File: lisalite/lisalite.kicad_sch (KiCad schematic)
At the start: 16 parts, among them J1 LisaLite FDD Connector, J2 LisaLite Twiggy Port Connector, U1 5MHz XTAL, U2 74LS74, U3 74LS393, U4 74LS85, U5 74LS85, U6 74LS164

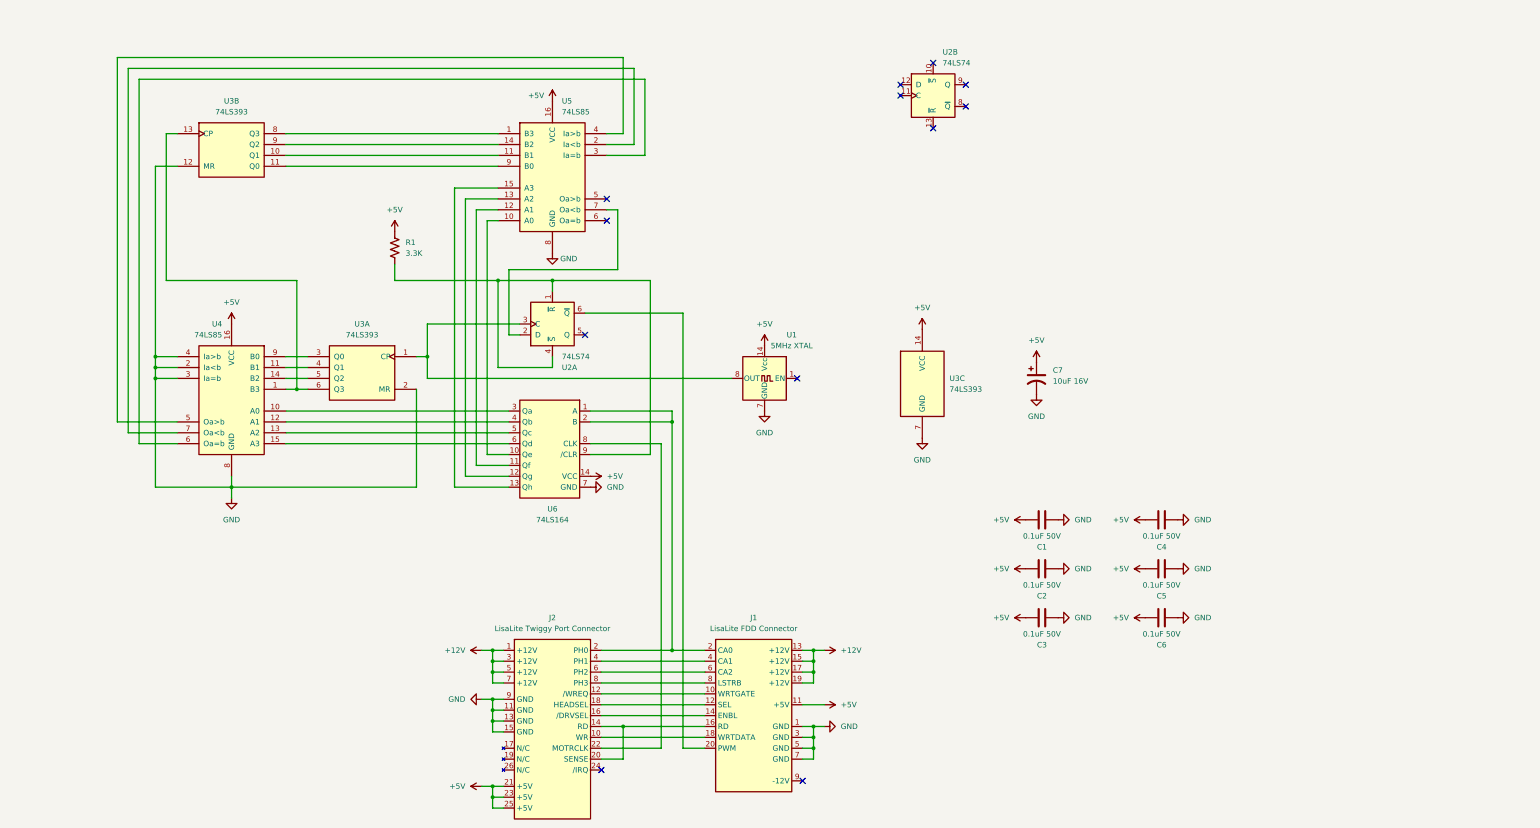
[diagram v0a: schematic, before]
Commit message: final commit for rev 1.0
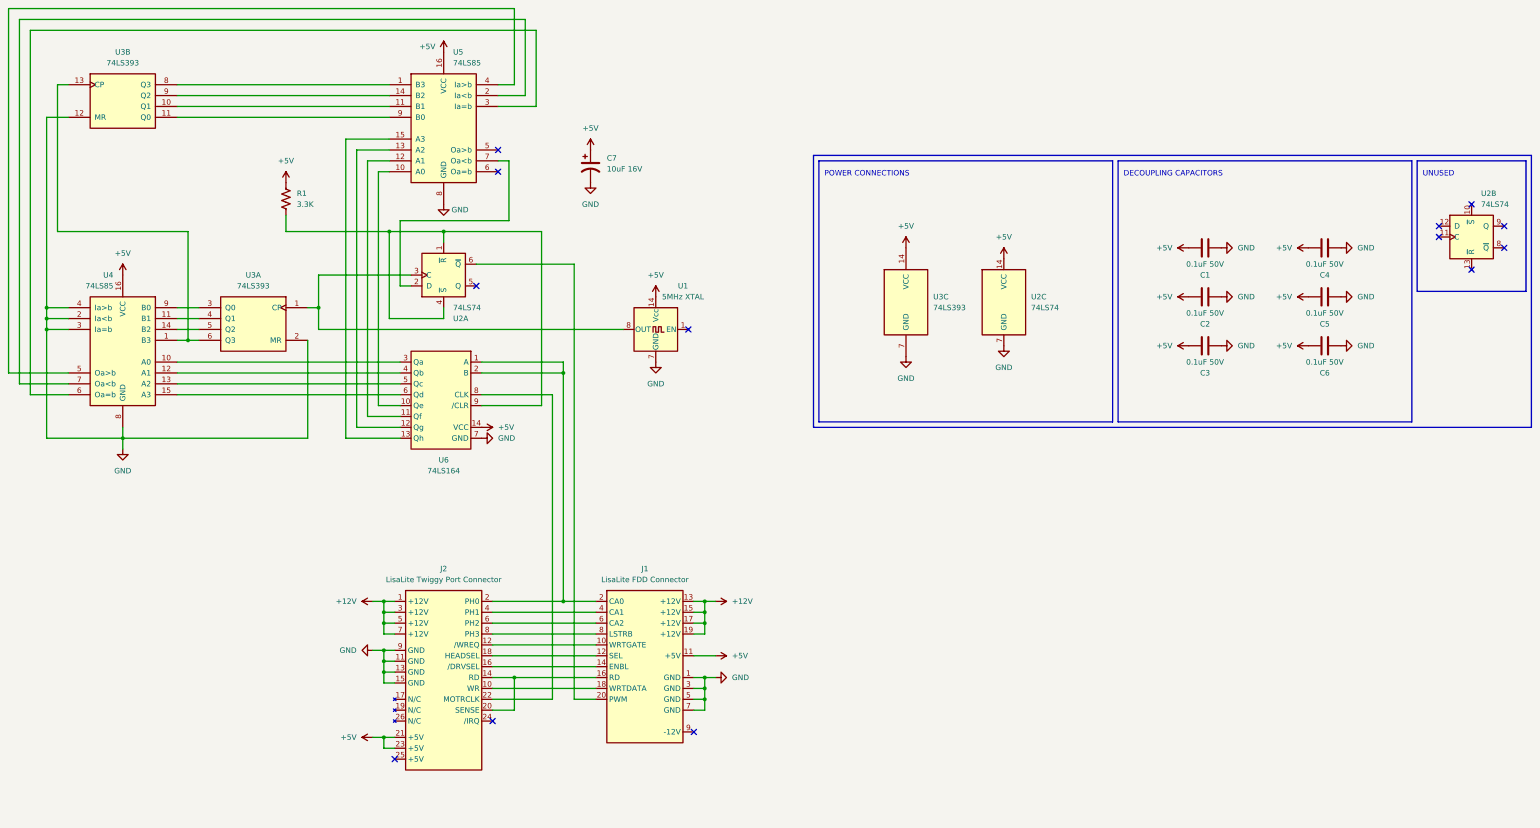
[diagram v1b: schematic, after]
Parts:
- added unit 3 of U2
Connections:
- net +5V: now also U2.14 (VCC); no longer J2.25 (+5V)
- net GND: now also U2.7 (GND)
- no-connect marks 12 -> 13
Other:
- note added: "DECOUPLING CAPACITORS"
- note added: "POWER CONNECTIONS"
- note added: "UNUSED"
- title: (none) -> Lisa Lite Adaptor
- moved on the sheet: C1, C2, C3, C4, C5, C6, C7, J1, J2, R1, U1, U2A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
